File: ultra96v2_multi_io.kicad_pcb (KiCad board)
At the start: 2 copper layers, 85 x 54 mm, 86 parts, among them J1 TE 5179030-2, J2 57202-G52-20LF, J3 1-1734248-5, J4 1-1734248-5, J5 PMOD, J6 PMOD, J7 PinHeader, J8 Conn_01x04, Q1 DMN63D8LDW-7, Q2 DMN63D8LDW-7, Q3 DMN63D8LDW-7, SW1 KMR213G LFG, SW2 KMR213G LFG, SW3 KMR213G LFG, SW4 KMR213G LFG, SW5 GDH04S04, U1 TPS62160DGK, U2 TXS0108EPW, U3 TXS0108EPW, U4 TXS0108EPW, U5 TXS0108EPW, U6 TXS0108EPW, X1 SIT2024BA-S3-18E-25.000000G, X2 <xxxMHz>

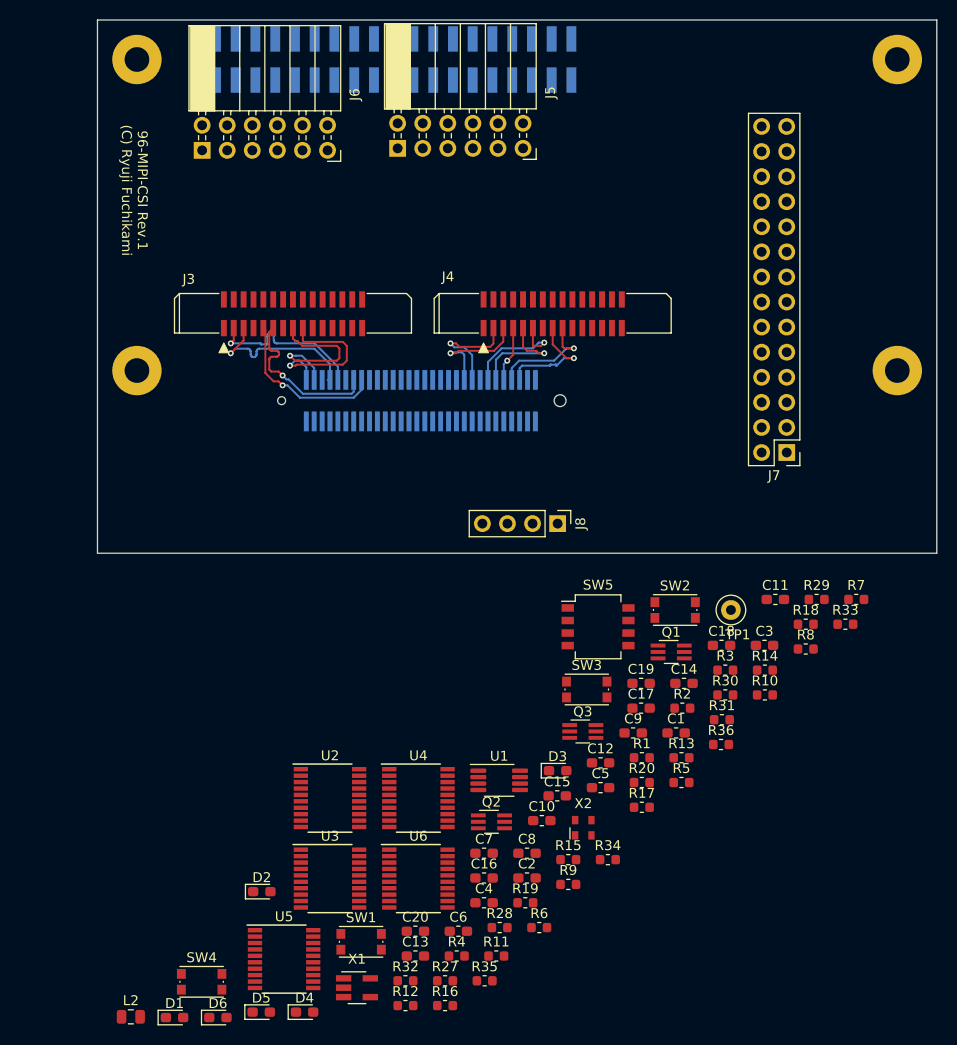
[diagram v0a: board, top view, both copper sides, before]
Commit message: update
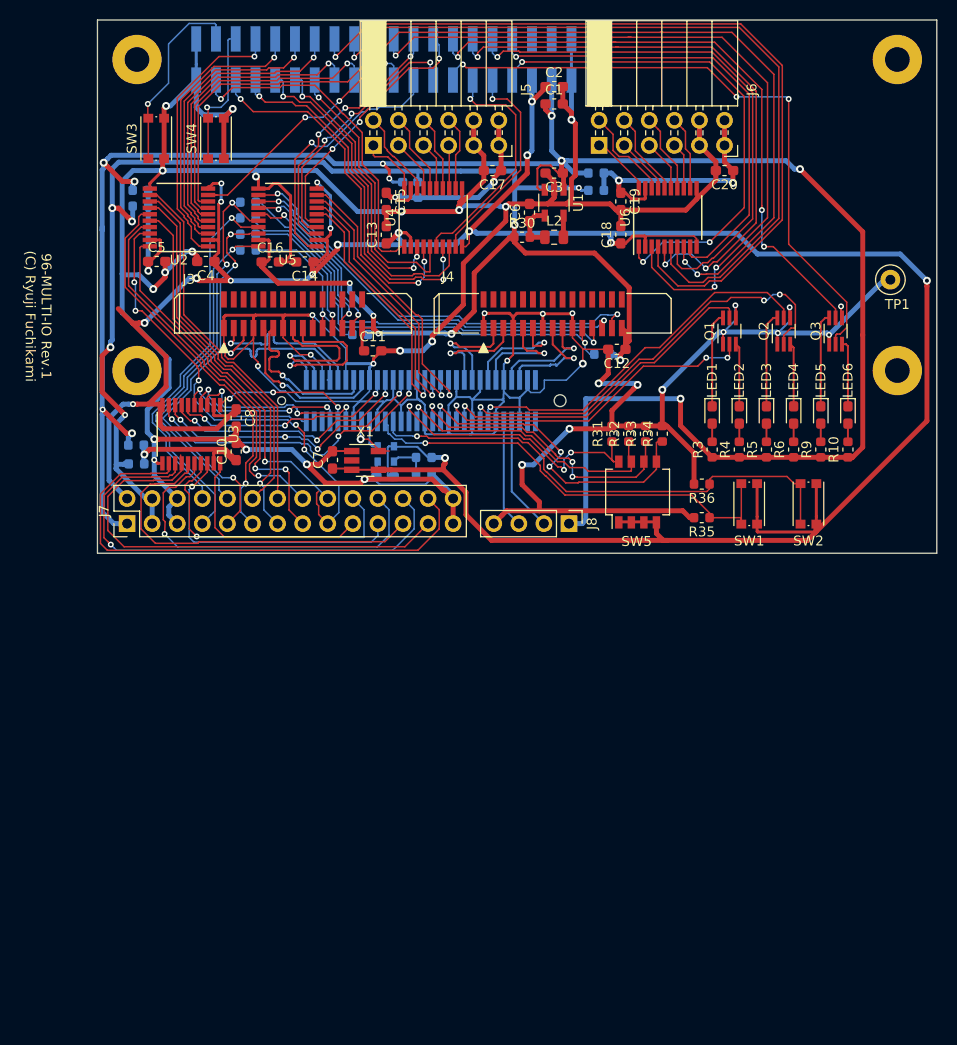
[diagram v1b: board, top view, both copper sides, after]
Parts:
- removed D2, D4, D5, D6: SML-512MWT86, LED_SMD:LED_0603_1608Metric_Pad1.05x0.95mm_HandSolder
- removed R27: 100k, Resistor_SMD:R_0603_1608Metric
- removed R28: 562k, Resistor_SMD:R_0603_1608Metric
- removed R29: 180k, Resistor_SMD:R_0603_1608Metric
- added LED2: SML-512MWT86, LED_SMD:LED_0603_1608Metric_Pad1.05x0.95mm_HandSolder, F.Cu at (165.0, 140.0)
- added LED4: SML-512MWT86, LED_SMD:LED_0603_1608Metric_Pad1.05x0.95mm_HandSolder, F.Cu at (170.5, 140.0)
- added LED5: SML-512MWT86, LED_SMD:LED_0603_1608Metric_Pad1.05x0.95mm_HandSolder, F.Cu at (173.2, 140.0)
- added LED6: SML-512MWT86, LED_SMD:LED_0603_1608Metric_Pad1.05x0.95mm_HandSolder, F.Cu at (176.0, 140.0)
- added R21: 0, Resistor_SMD:R_0603_1608Metric, B.Cu at (126.6, 131.8)
- added R22: 0, Resistor_SMD:R_0603_1608Metric, B.Cu at (151.1, 133.8)
- C3: value 10uF -> 4.7uF
- C6: value 22uF -> 10uF
- C9, R1, R11, R12, R13, R14, R19, R2, R20, R7, R8, X2: moved to B.Cu
- R15, R16, R17, R18: value 0 -> <0>; moved to B.Cu
- U1: value TPS62160DGK -> LM3671MF-3.3/NOPB; footprint myfootprint:TPS62160DGK -> Package_TO_SOT_SMD:TSOT-23-5
- moved L2 89.8 mm to (146.2, 122.0)
- moved SW4 85.4 mm to (112.0, 112.0), turned to 90 degrees
- moved C20 83.1 mm to (163.5, 115.2), turned to 180 degrees
- moved LED1 81.8 mm to (162.2, 140.0), turned to 270 degrees
- moved R16 80.6 mm to (115.2, 121.7), turned to 180 degrees
- moved C2 80.2 mm to (146.2, 106.8)
- moved R2 75.9 mm to (104.3, 117.2), turned to 180 degrees
- moved R1 75.5 mm to (104.3, 118.8), turned to 180 degrees
- moved U5 75.1 mm to (119.2, 120.0), turned to 180 degrees
- moved C6 73.1 mm to (143.8, 119.5), turned to 90 degrees
- moved C13 73.1 mm to (129.2, 121.8), turned to 90 degrees
- moved R19 72.5 mm to (150.5, 117.2), turned to 180 degrees
- moved R17 71.8 mm to (115.2, 120.0), turned to 180 degrees
- moved U6 71.6 mm to (157.8, 120.0), turned to 90 degrees
- moved R18 70.8 mm to (115.2, 118.5), turned to 180 degrees
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- renumbered D1 to LED1, D3 to LED3
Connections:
- J5 pad 6: +3V3 -> /PMOD1_VDD
- J6 pad 6: +3V3 -> /PMOD2_VDD
- SW5 pad 1: /HS_DSI_D0_P -> +1V8
- SW5 pad 2: /HS_DSI_D0_N -> +1V8
- SW5 pad 3: /HS_DSI_D1_P -> +1V8
- SW5 pad 4: /HS_DSI_D1_N -> +1V8
- SW5 pad 5: +1V8 -> /HS_DSI_D1_N
- SW5 pad 6: +1V8 -> /HS_DSI_D1_P
- SW5 pad 7: +1V8 -> /HS_DSI_D0_N
- SW5 pad 8: +1V8 -> /HS_DSI_D0_P
- U1 pad 1: GND -> +5V
- U1 pad 2: +5V -> GND
- U1 pad 4: GND -> Net-(C6-Pad1)
- U1 pad 5: Net-(R28-Pad1) -> Net-(L2-Pad2)
- U4 pad 13: /PMOD1_9 -> /PMOD1_4
- U4 pad 14: /PMOD1_8 -> /PMOD1_9
- U4 pad 15: /PMOD1_7 -> /PMOD1_3
- U4 pad 16: /PMOD1_4 -> /PMOD1_8
- U4 pad 17: /PMOD1_3 -> /PMOD1_2
- U4 pad 18: /PMOD1_2 -> /PMOD1_7
- U4 pad 3: /LS_GPIO_1 -> /LS_GPIO_4
- U4 pad 4: /LS_GPIO_2 -> /LS_GPIO_1
- U4 pad 5: /LS_GPIO_3 -> /LS_GPIO_5
- U4 pad 6: /LS_GPIO_4 -> /LS_GPIO_6
- U4 pad 7: /LS_GPIO_5 -> /LS_GPIO_2
- U4 pad 8: /LS_GPIO_6 -> /LS_GPIO_3
- U6 pad 13: /PMOD2_9 -> /PMOD2_4
- U6 pad 14: /PMOD2_8 -> /PMOD2_9
- U6 pad 15: /PMOD2_7 -> /PMOD2_3
- U6 pad 16: /PMOD2_4 -> /PMOD2_8
- U6 pad 17: /PMOD2_3 -> /PMOD2_2
- U6 pad 18: /PMOD2_2 -> /PMOD2_7
- U6 pad 3: /LS_GPIO_9 -> /LS_GPIO_12
- U6 pad 4: /LS_GPIO_10 -> /LS_GPIO_9
- U6 pad 5: /LS_GPIO_11 -> /LS_GPIO_13
- U6 pad 6: /LS_GPIO_12 -> /LS_GPIO_10
- U6 pad 7: /LS_GPIO_13 -> /LS_GPIO_14
- U6 pad 8: /LS_GPIO_14 -> /LS_GPIO_11
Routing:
- net GND: track 5.71 -> 555.2 mm, vias 1 -> 38
- net +1V8: track 0.00 -> 312.3 mm, vias 0 -> 17
- net +5V: track 0.00 -> 227.1 mm, vias 0 -> 10
- net +3V3: track 0.00 -> 172.9 mm, vias 0 -> 11
- net /LS_GPIO_9: track 0.00 -> 84.0 mm, vias 0 -> 1
- net /LS_GPIO_10: track 0.00 -> 79.3 mm, vias 0 -> 1
- net /LS_GPIO_12: track 0.00 -> 74.9 mm, vias 0 -> 3
- net /LS_GPIO_11: track 0.00 -> 73.3 mm, vias 0 -> 3
- net /LS_PS_GPIO_4: track 0.00 -> 64.5 mm, vias 0 -> 3
- net /LS_PS_GPIO_5: track 0.00 -> 62.8 mm, vias 0 -> 3
- net /LS_GPIO_13: track 0.00 -> 61.3 mm, vias 0 -> 3
- net /LS_GPIO_14: track 0.00 -> 54.4 mm, vias 0 -> 1
- net /PH_GPIO_D: track 0.00 -> 52.7 mm
- net /LS_GPIO_8: track 0.00 -> 51.7 mm, vias 0 -> 3
- net /HS_DSI_CLK_N: track 0.00 -> 51.1 mm, vias 0 -> 1
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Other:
- board text added: "96-MULTI-IO Rev.1 (C) Ryuji Fuchikami"
- board text removed: "96-MIPI-CSI Rev.1 (C) Ryuji Fuchikami"
